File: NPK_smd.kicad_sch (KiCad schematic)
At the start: 57 parts, among them J1 DHT, J2 Screw_Terminal_01x04, J3 USB_C_Receptacle_USB2.0_16P, J4 Conn_01x02_Pin, Q3 SS8050, Q4 SS8050, SW1 SW_Push, SW2 SW_Push, SW3 SW_SPST, U1 AMS1117-3.3, U2 MAX485ESA_T, U3 LM2596S-ADJ, U4 ESP32-WROOM-32, U6 USBLC6-2SC6, U7 CH340C

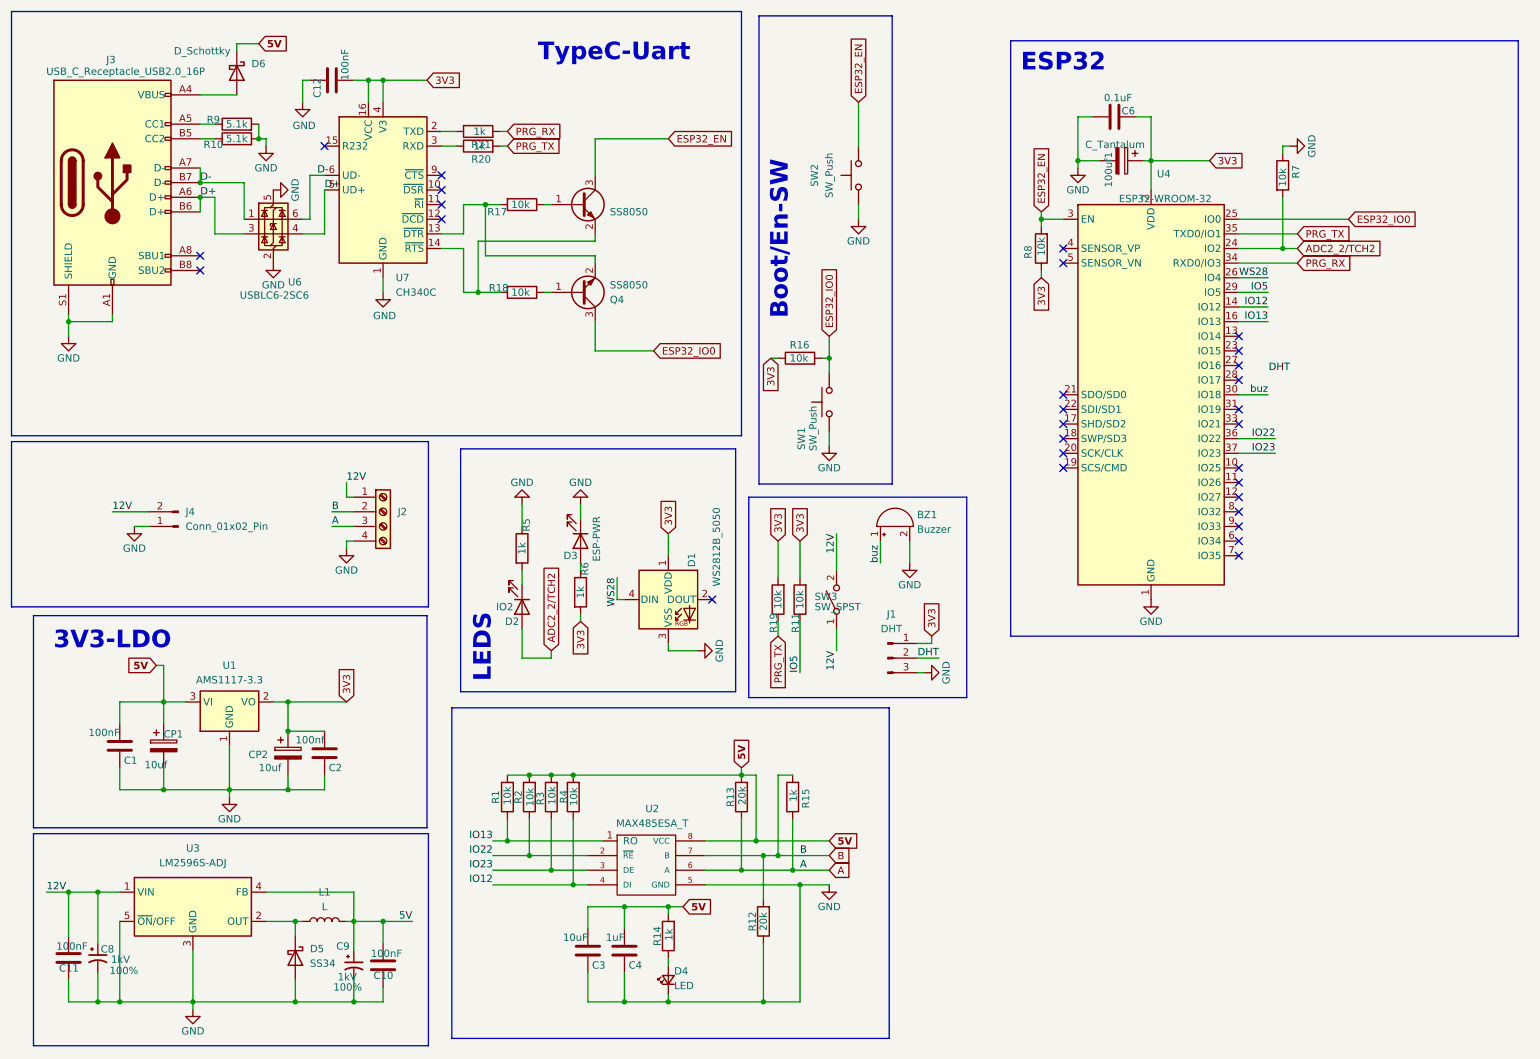
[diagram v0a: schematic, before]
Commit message: version-1.0 rev 2026-04-11
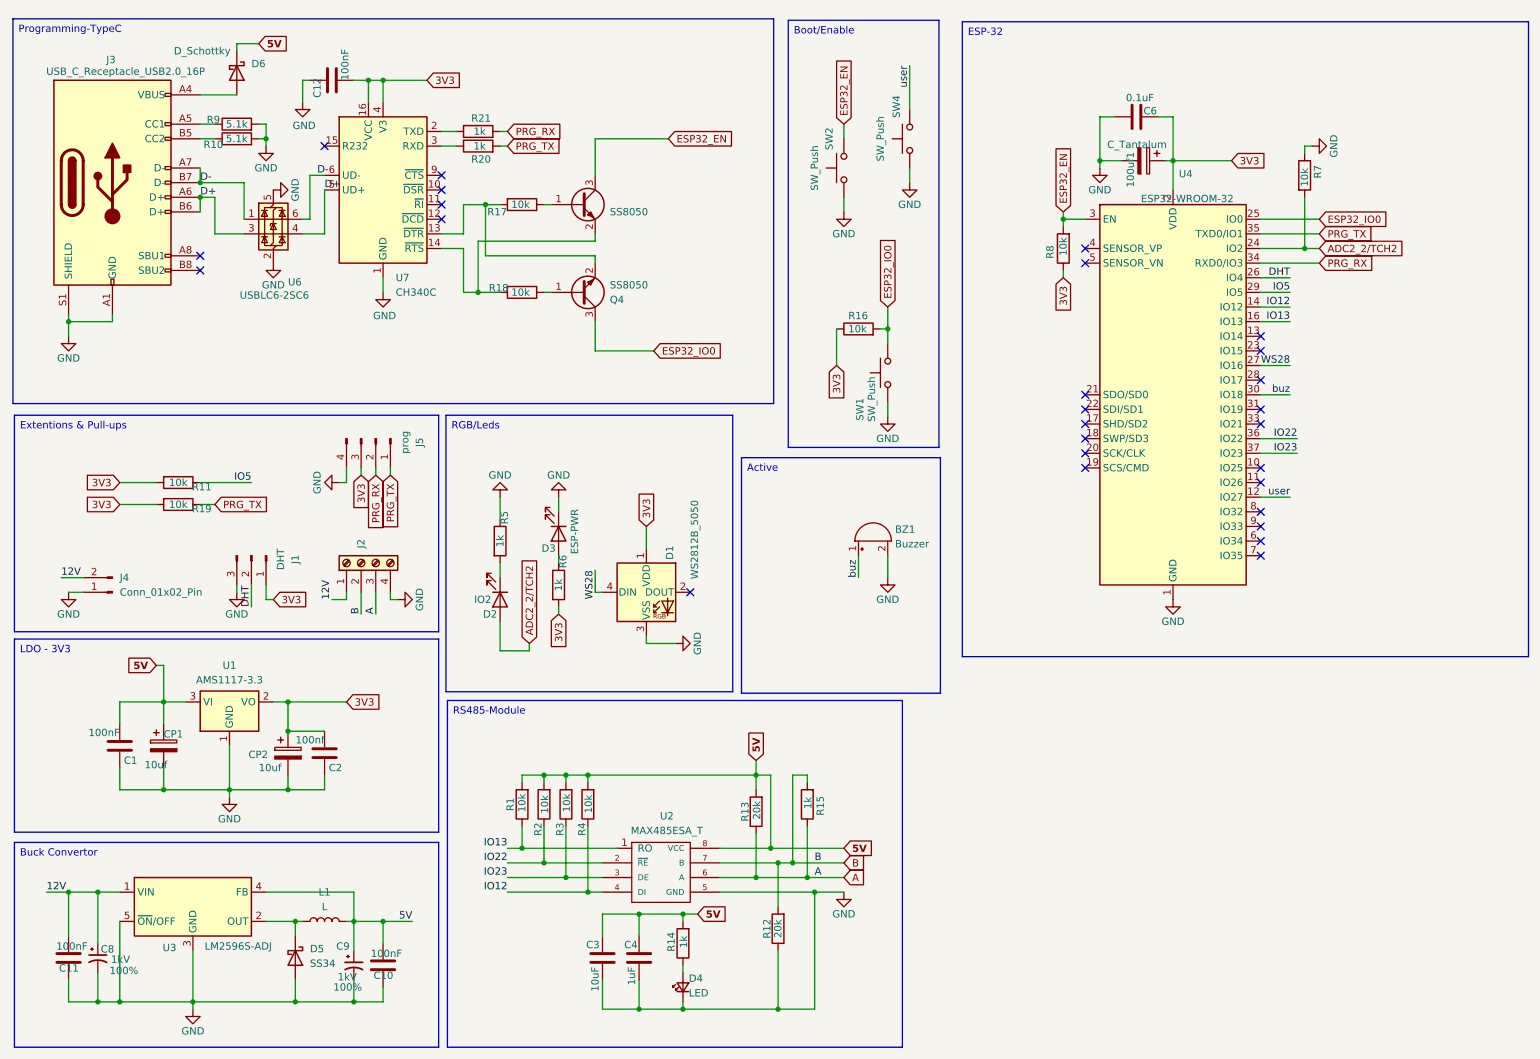
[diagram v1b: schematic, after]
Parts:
- removed SW3: SW_SPST, TestPoint:TestPoint_2Pads_Pitch2.54mm_Drill0.8mm, symbol Switch:SW_SPST
- added J5: prog, Connector_PinHeader_2.54mm:PinHeader_1x04_P2.54mm_Vertical_SMD_Pin1Left, symbol Connector:Conn_01x04_Pin
- added SW4: SW_Push, tactile-switch:SW_B3U-1000PM, symbol Switch:SW_Push
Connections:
- net 3V3: now also J5.3 (Pin_3)
- net DHT: now also U4.26 (IO4)
- net GND: now also J5.4 (Pin_4), SW4.1
- net PRG_RX: now also J5.2 (Pin_2)
- net PRG_TX: now also J5.1 (Pin_1)
- net WS28: now also U4.27 (IO16); no longer U4.26 (IO4)
- net user: now reaches U4.12 (IO27)
- net user: now also SW4.2
- no-connect marks 29 -> 27
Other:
- note removed: "3V3-LDO"
- note removed: "Boot/En-SW"
- note removed: "ESP32"
- note removed: "LEDS"
- note removed: "TypeC-Uart"
- company: (none) -> AR RoboTics
- title: (none) -> Bhoomitra
- moved on the sheet: 100uf1, BZ1, C3, C4, C6, D1, D2, D3, D4, J1, J2, J4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
